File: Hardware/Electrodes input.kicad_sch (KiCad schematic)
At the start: 47 parts, among them J2 Conn_01x26_Pin, U2 TPD4E1B06DRLR

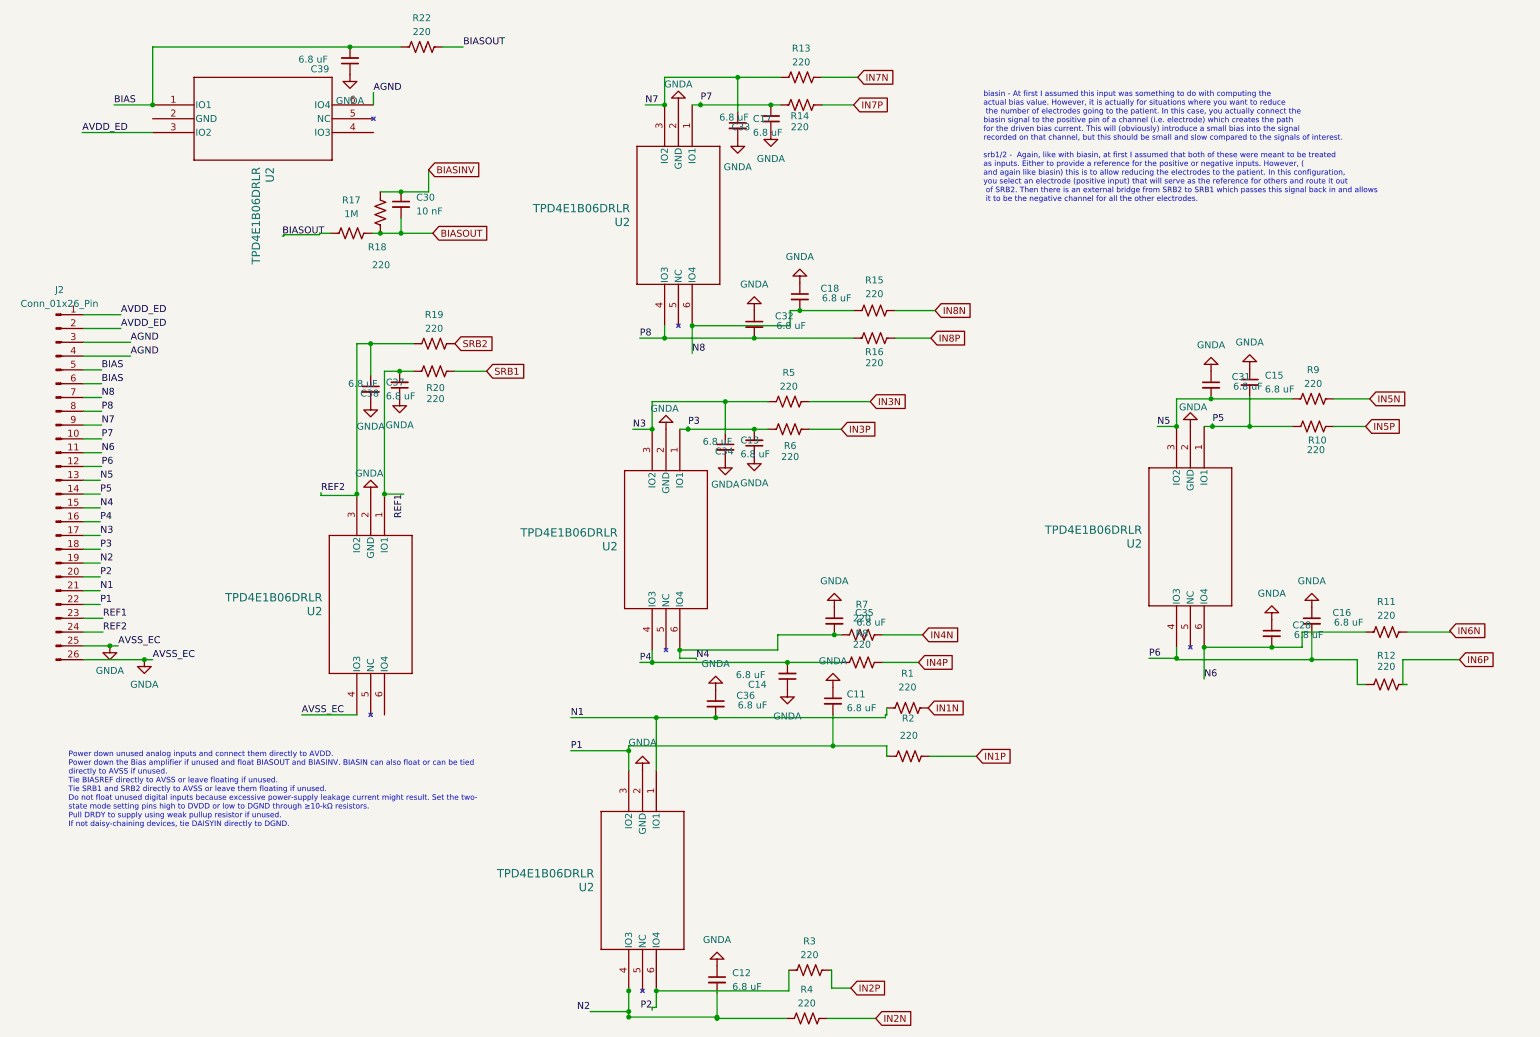
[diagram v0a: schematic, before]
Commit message: DIY_EEG board design changes
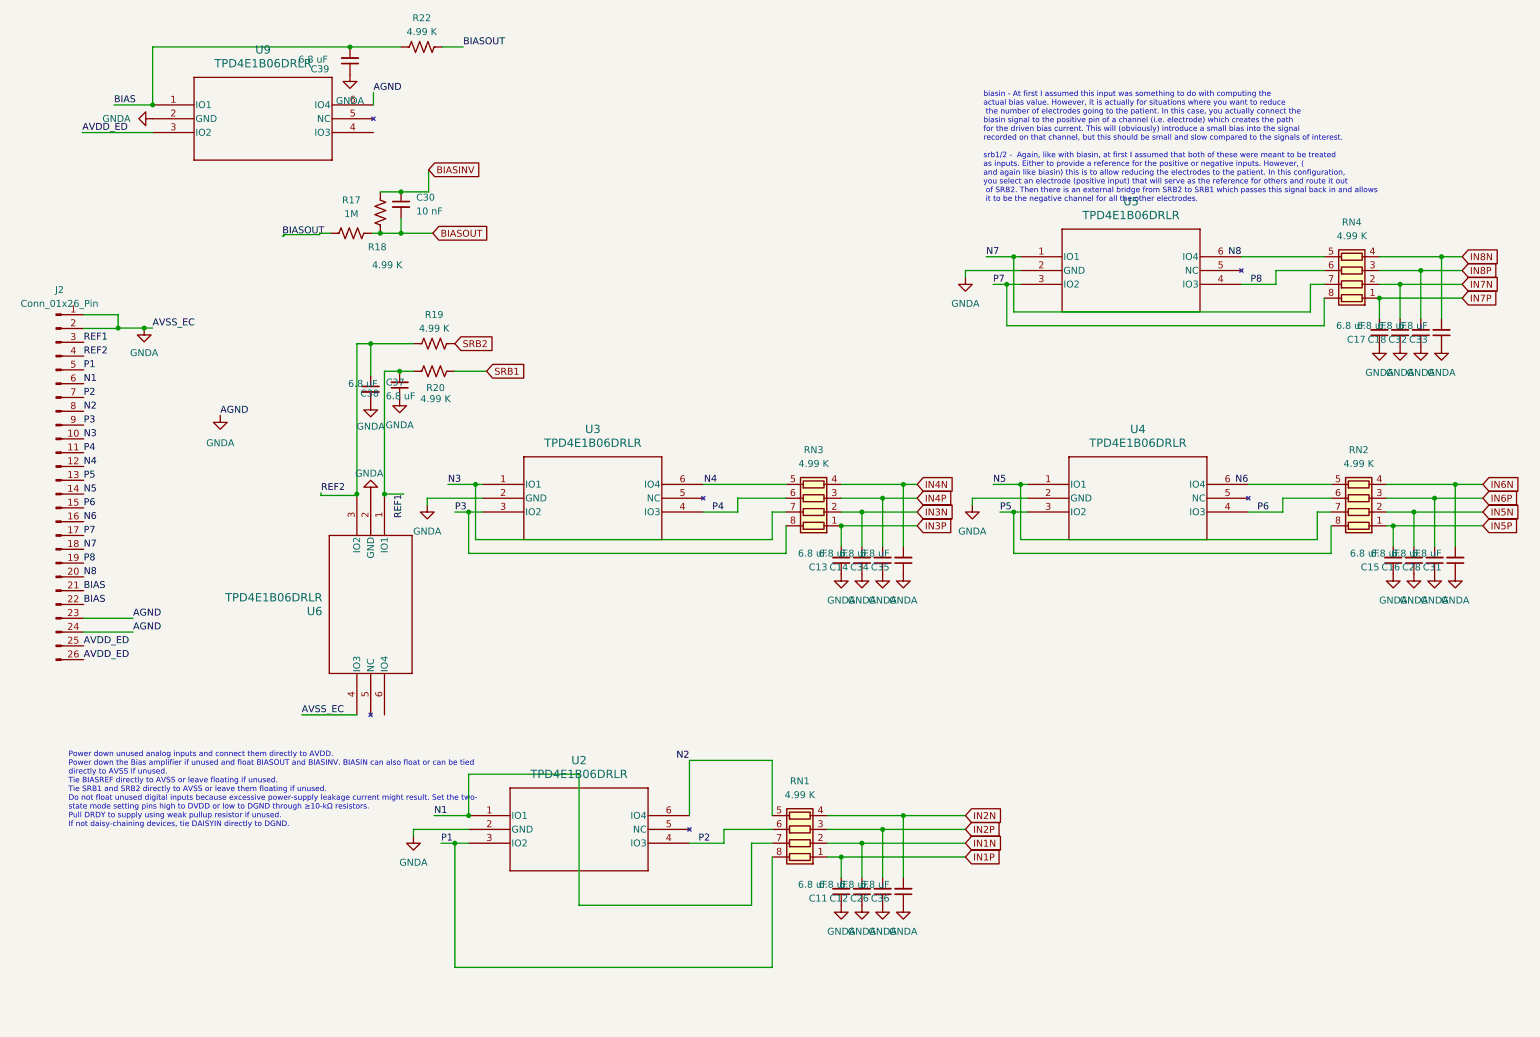
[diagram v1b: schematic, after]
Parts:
- removed R1, R10, R11, R12, R13, R14, R15, R16, R2, R3, R4, R5, R6, R7, R8, R9: 220, Resistor_SMD:R_0603_1608Metric, symbol Device:R_US
- removed U2 (x3): TPD4E1B06DRLR, ESD:DRL6_TEX, symbol 2024-02-26_11-45-18:TPD4E1B06DRLR
- added C26: 6.8 uF, Capacitor_SMD:C_0201_0603Metric, symbol Device:C_Small
- added RN1, RN2, RN3, RN4: 4.99 K, Resistor_SMD:R_Array_Convex_4x0402, symbol Device:R_Pack04
- added U3, U4, U5: TPD4E1B06DRLR, tpd4e1b06:DRL6_TEX, symbol 2024-02-26_11-45-18:TPD4E1B06DRLR
- C11, C12, C13, C14, C15, C16, C17, C18, C28, C31, C32, C33, C34, C35, C36, C37, C38, C39: footprint Capacitor_SMD:C_0603_1608Metric_Pad1.08x0.95mm_HandSolder -> Capacitor_SMD:C_0201_0603Metric
- C30: footprint (none) -> Capacitor_SMD:C_0201_0603Metric
- J2: footprint (none) -> Connector_PinHeader_2.54mm:PinHeader_2x13_P2.54mm_Horizontal
- R17: footprint Resistor_SMD:R_0603_1608Metric -> Resistor_SMD:R_0201_0603Metric
- R18, R19, R20, R22: value 220 -> 4.99 K; footprint Resistor_SMD:R_0603_1608Metric -> Resistor_SMD:R_0201_0603Metric
- U2: footprint ESD:DRL6_TEX -> tpd4e1b06:DRL6_TEX
- U6, U9: renamed from U2; footprint ESD:DRL6_TEX -> tpd4e1b06:DRL6_TEX
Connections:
- net AVDD_ED: now also J2.25 (Pin_25), J2.26 (Pin_26); no longer J2.1 (Pin_1), J2.2 (Pin_2)
- net BIAS: now also J2.21 (Pin_21), J2.22 (Pin_22); no longer J2.5 (Pin_5), J2.6 (Pin_6)
- net GNDA: now also C13.1, C17.1, J2.1 (Pin_1), J2.2 (Pin_2), J2.23 (Pin_23), J2.24 (Pin_24), U9.2 (GND), U9.6 (IO4), C26.1, U3.2 (GND), U4.2 (GND), U5.2 (GND); no longer C13.2, C17.2, J2.25 (Pin_25), J2.26 (Pin_26)
- net IN1N: now also C12.2, RN1.2 (R2.1)
- net IN1P: now also C11.2, RN1.1 (R1.1)
- net IN2N: now also C36.2, RN1.4 (R4.1)
- net IN2P: now also C26.2, RN1.3 (R3.1)
- net IN3N: now also C14.2, RN3.2 (R2.1)
- net IN3P: now also C13.2, RN3.1 (R1.1)
- net IN4N: now also C35.2, RN3.4 (R4.1)
- net IN4P: now also C34.2, RN3.3 (R3.1)
- net IN5N: now also C16.2, RN2.2 (R2.1)
- net IN5P: now also C15.2, RN2.1 (R1.1)
- net IN6N: now also C31.2, RN2.4 (R4.1)
- net IN6P: now also C28.2, RN2.3 (R3.1)
- net IN7N: now also C18.2, RN4.2 (R2.1)
- net IN7P: now also C17.2, RN4.1 (R1.1)
- net IN8N: now also C33.2, RN4.4 (R4.1)
- net IN8P: now also C32.2, RN4.3 (R3.1)
- net N1: now also J2.6 (Pin_6), RN1.7 (R2.2); no longer C36.2, J2.21 (Pin_21)
- net N2: now also J2.8 (Pin_8), U2.6 (IO4), RN1.5 (R4.2); no longer C12.2, J2.19 (Pin_19), U2.4 (IO3)
- net N3: now also J2.10 (Pin_10), RN3.7 (R2.2), U3.1 (IO1); no longer C13.1, J2.17 (Pin_17)
- net N4: now also J2.12 (Pin_12), RN3.5 (R4.2), U3.6 (IO4); no longer C35.2, J2.15 (Pin_15)
- net N5: now also J2.14 (Pin_14), RN2.7 (R2.2), U4.1 (IO1); no longer C31.2, J2.13 (Pin_13)
- net N6: now also J2.16 (Pin_16), RN2.5 (R4.2), U4.6 (IO4); no longer C28.2, J2.11 (Pin_11)
- net N7: now also J2.18 (Pin_18), RN4.7 (R2.2), U5.1 (IO1); no longer C17.1, J2.9 (Pin_9)
- net N8: now also J2.20 (Pin_20), RN4.5 (R4.2), U5.6 (IO4); no longer C18.2, J2.7 (Pin_7)
- net P1: now also J2.5 (Pin_5), RN1.8 (R1.2); no longer C11.2, J2.22 (Pin_22)
- net P2: now also J2.7 (Pin_7), U2.4 (IO3), RN1.6 (R3.2); no longer J2.20 (Pin_20), U2.6 (IO4)
- net P3: now also J2.9 (Pin_9), RN3.8 (R1.2), U3.3 (IO2); no longer C34.2, J2.18 (Pin_18)
- net P4: now also J2.11 (Pin_11), RN3.6 (R3.2), U3.4 (IO3); no longer C14.2, J2.16 (Pin_16)
- net P5: now also J2.13 (Pin_13), RN2.8 (R1.2), U4.3 (IO2); no longer C15.2, J2.14 (Pin_14)
- net P6: now also J2.15 (Pin_15), RN2.6 (R3.2), U4.4 (IO3); no longer C16.2, J2.12 (Pin_12)
- net P7: now also J2.17 (Pin_17), RN4.8 (R1.2), U5.3 (IO2); no longer C33.2, J2.10 (Pin_10)
- net P8: now also J2.19 (Pin_19), RN4.6 (R3.2), U5.4 (IO3); no longer C32.2, J2.8 (Pin_8)
- net REF1: now also J2.3 (Pin_3); no longer J2.23 (Pin_23)
- net REF2: now also J2.4 (Pin_4); no longer J2.24 (Pin_24)
- removed net AGND: J2.3 (Pin_3), J2.4 (Pin_4), U9.6 (IO4)
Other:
- moved on the sheet: U2
